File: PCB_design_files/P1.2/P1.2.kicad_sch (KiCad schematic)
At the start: 37 parts, among them J1 -EEG_INPUT, J2 +EEG_INPUT, J3 +3.3V, J4 GND, J5 -3V3, J6 EEG_INPUT, J7 STAGE_1_OUT, J8 STAGE_2_OUT, J9 STAGE_3_OUT, U1 INA819, U2 TPS61094, U3 TLV9102, U4 TC1044

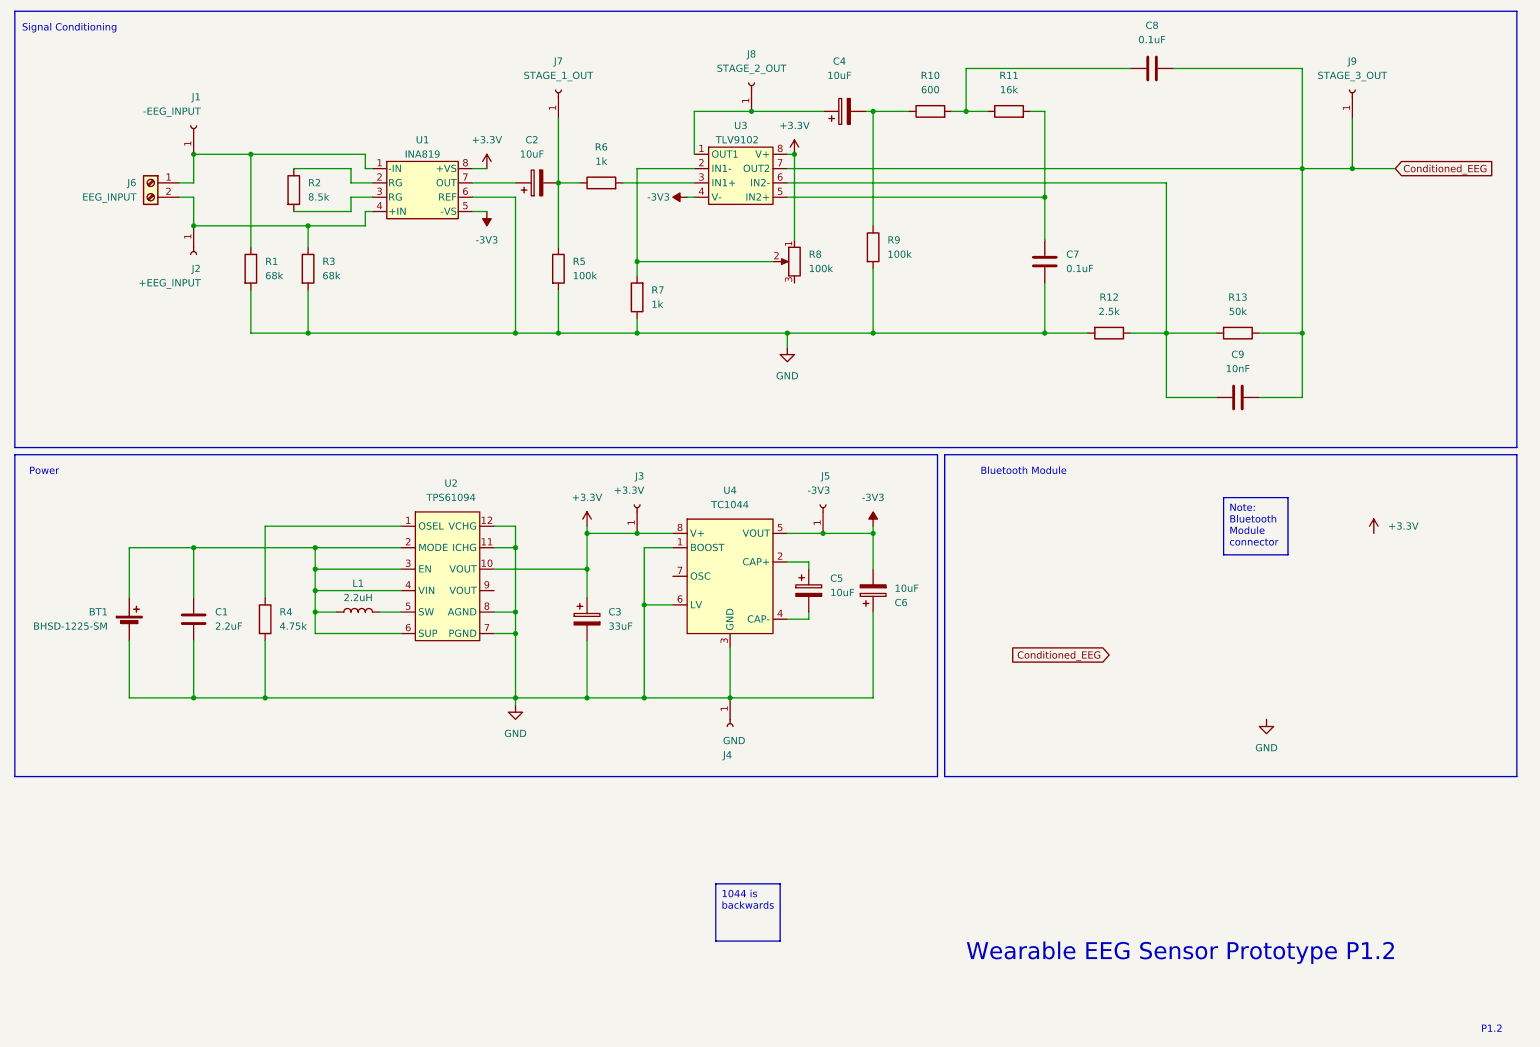
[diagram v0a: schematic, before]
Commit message: Created PCB Layout
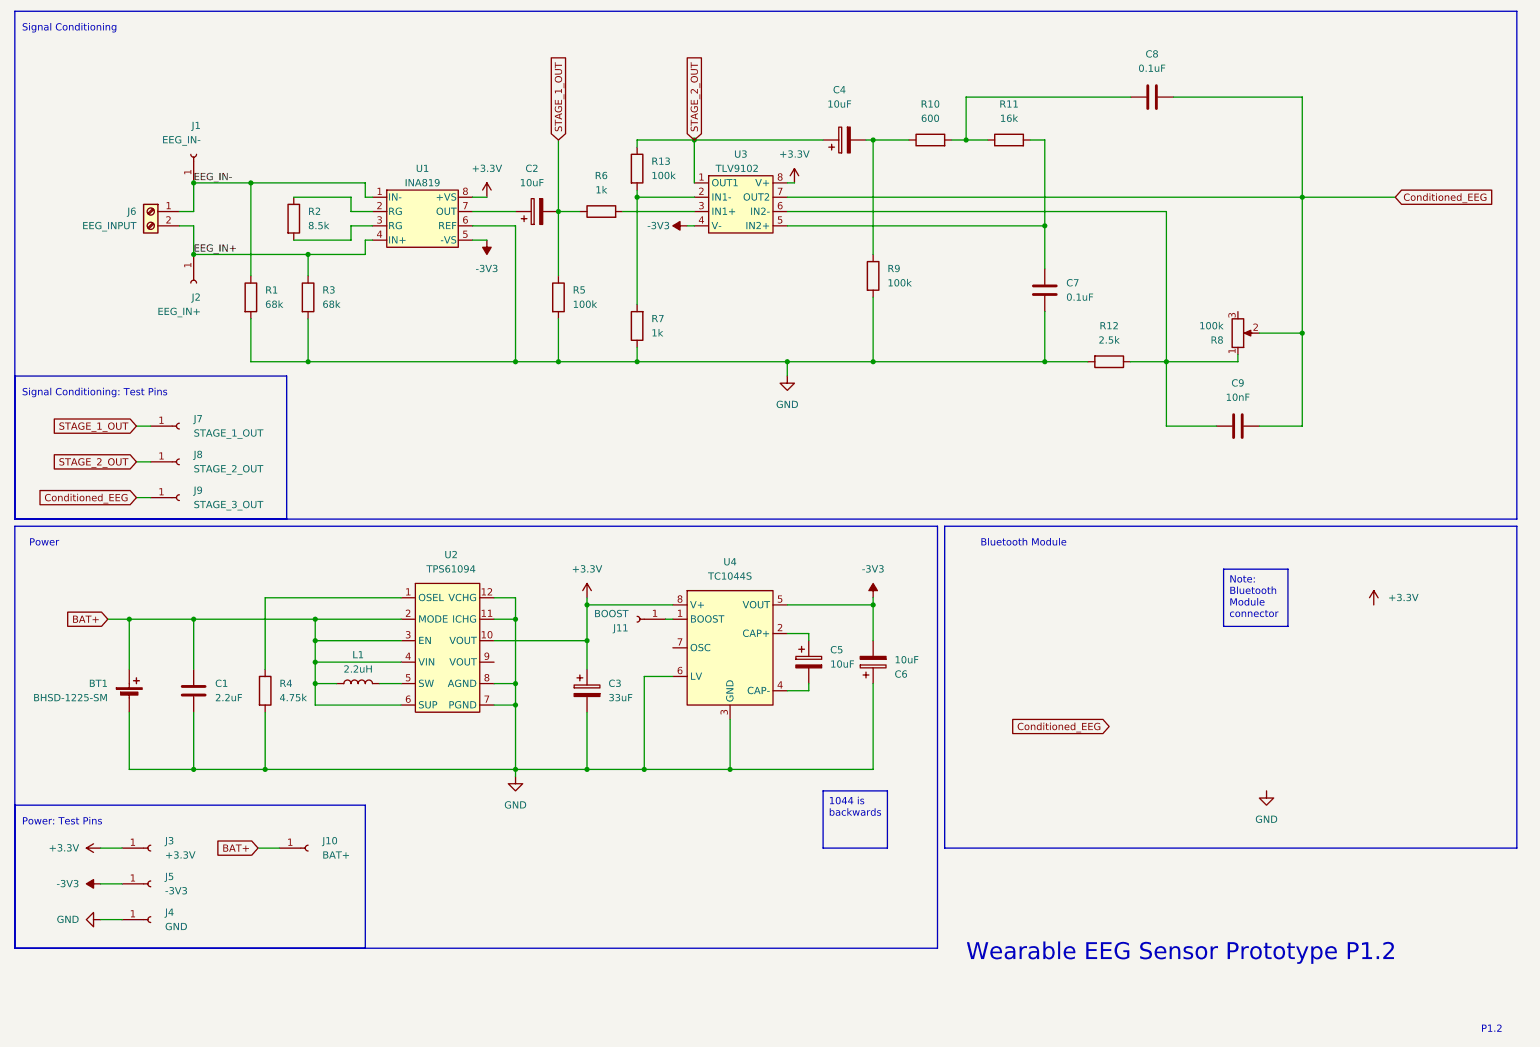
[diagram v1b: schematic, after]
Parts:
- added J10: BAT+, TestPoint:TestPoint_Loop_D2.50mm_Drill1.0mm, symbol Connector:Conn_01x01_Socket
- added J11: BOOST, TestPoint:TestPoint_Loop_D2.50mm_Drill1.0mm, symbol Connector:Conn_01x01_Socket
- J1: value -EEG_INPUT -> EEG_IN-
- J2: value +EEG_INPUT -> EEG_IN+
- R13: value 50k -> 100k
- U4: value TC1044 -> TC1044S
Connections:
- net +3.3V: no longer R8.1
- net Conditioned_EEG: now also R8.2; no longer R13.1
- net GND: no longer U4.1 (BOOST)
- net at C9.2, R12.1, U3.6 (IN2-): now also R8.1; no longer R13.2
- net STAGE_2_OUT: now reaches C4.1, J8.1 (Pin_1), U3.1 (OUT1)
- net STAGE_2_OUT: now also R13.1
- net STAGE_1_OUT: now reaches C2.2, J7.1 (Pin_1), R5.1, R6.1
- net EEG_IN-: now reaches J1.1 (Pin_1), J6.1 (EEG_IN-), R1.1, U1.1 (IN-)
- net EEG_IN+: now reaches J2.1 (Pin_1), J6.2 (EEG_IN-), R3.1, U1.4 (IN+)
- net BAT+: now reaches BT1.1 (+), C1.1, L1.1, U2.2 (MODE), U2.3 (EN), U2.4 (VIN), U2.6 (SUP)
- net BAT+: now also J10.1 (Pin_1)
- net at R7.2, U3.2 (IN1-): now also R13.2; no longer R8.2
- new net: J11.1 (Pin_1), U4.1 (BOOST)
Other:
- note added: "Power: Test Pins"
- note added: "Signal Conditioning: Test Pins"
- moved on the sheet: BT1, C1, C2, C3, C4, C5, C6, C7, C8, C9, J1, J2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
